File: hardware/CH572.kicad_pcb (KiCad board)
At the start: 2 copper layers, 17.8 x 28.9 mm, 15 parts, among them J1 Conn_01x07, J4 USB_C_Receptacle_USB2.0_14P, J5 Conn_01x07, SW1 SW_Push, SW2 SW_Push, U1 CH572D, Y1 32MHz

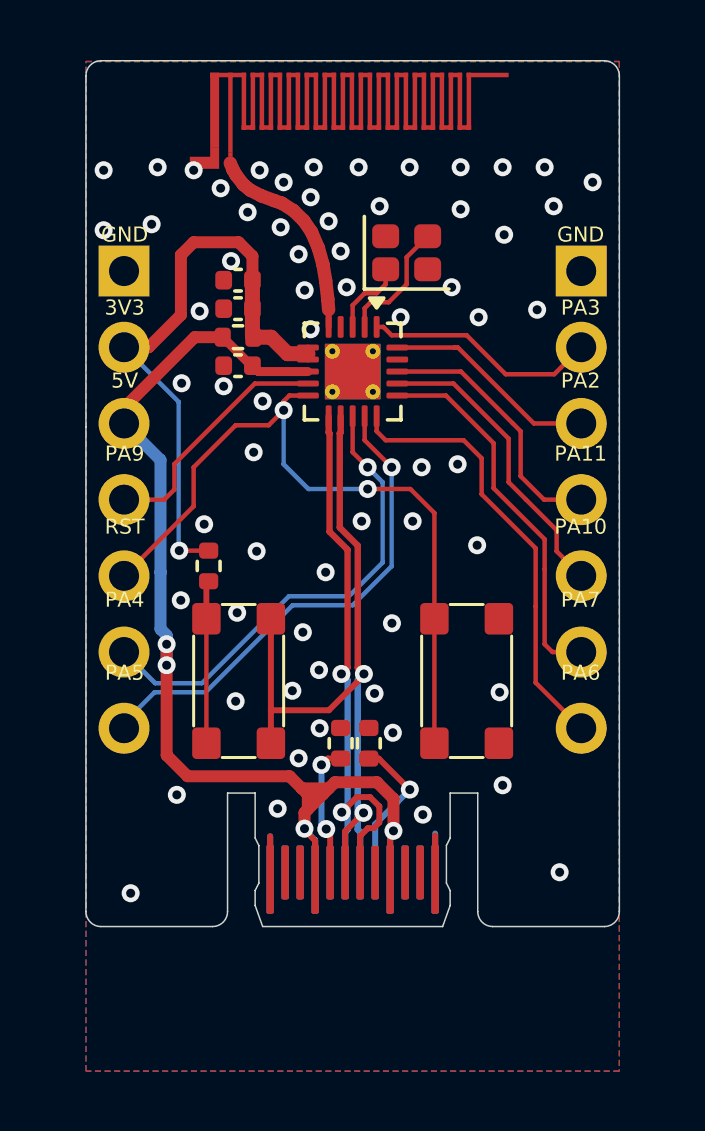
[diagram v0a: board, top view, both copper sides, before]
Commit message: Stash
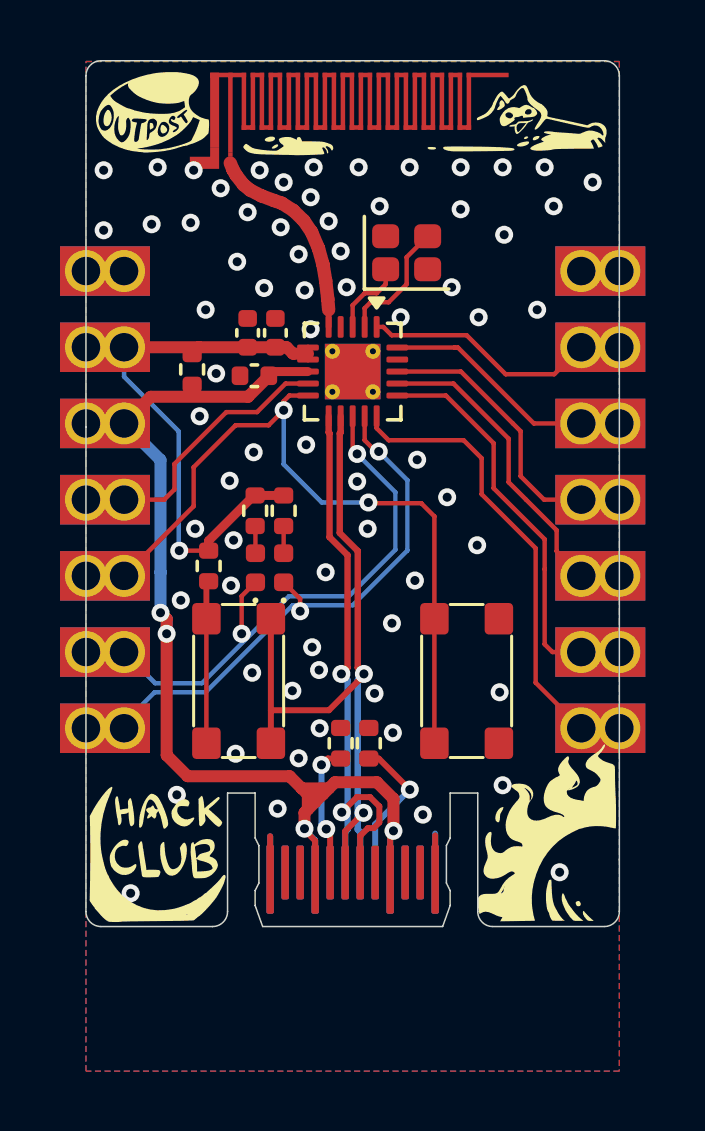
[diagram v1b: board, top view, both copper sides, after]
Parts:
- added D2: LED, LED_SMD:LED_0402_1005Metric, F.Cu at (111.1, 70.8)
- added D3: LED, LED_SMD:LED_0402_1005Metric, F.Cu at (112.0, 70.8)
- added G*** (x2): LOGO, LOGO, F.Cu at (114.6, 68.2)
- added G*** (x2): LOGO, LOGO, B.Cu at (114.0, 68.2)
- added R5: 1.5k, Resistor_SMD:R_0402_1005Metric, F.Cu at (111.0, 69.0)
- added R6: 1.5k, Resistor_SMD:R_0402_1005Metric, F.Cu at (112.0, 69.0)
- J1, J5: footprint Connector_PinHeader_2.54mm:PinHeader_1x07_P2.54mm_Vertical -> PCM_ckl-castellated-2.54mm:Castellated_1x07_P2.54mm_Vertical
- moved R1 1.87 mm to (109.0, 64.2), turned to -90 degrees
- moved C2 1.78 mm to (110.8, 63.0), turned to 90 degrees
- moved C3 1.48 mm to (111.7, 63.0), turned to 90 degrees
- moved C1 0.64 mm to (111.0, 64.5)
- moved J1 0.64 mm to (106.0, 76.2)
- moved J5 0.64 mm to (122.6, 76.2)
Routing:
- net /PA4: track 16.0 -> 18.3 mm, vias 1 -> 2
- net +3V3: track 21.3 -> 19.4 mm
- net /PA5: track 16.6 -> 18.3 mm, vias 1 -> 2
- net +5V: track 40.2 -> 39.0 mm
- net Net-(D2-A): track 0.00 -> 0.91 mm
- net Net-(D3-A): track 0.00 -> 0.91 mm
- net GND: vias 64 -> 69
